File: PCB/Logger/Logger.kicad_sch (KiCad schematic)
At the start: 78 parts, among them J2 USB-C-Socket-V, J3 JST-PH-SM4-TB, J4 Reset, J5 Conn_01x05, J6 TF_PUSH, J7 TC2030-USB-NL-DS, Q1 C179347, Q4 CJ2301, U1 TP4054, U10 ESP32-S3-MINI-1, U2 ME6211C33M5G-N

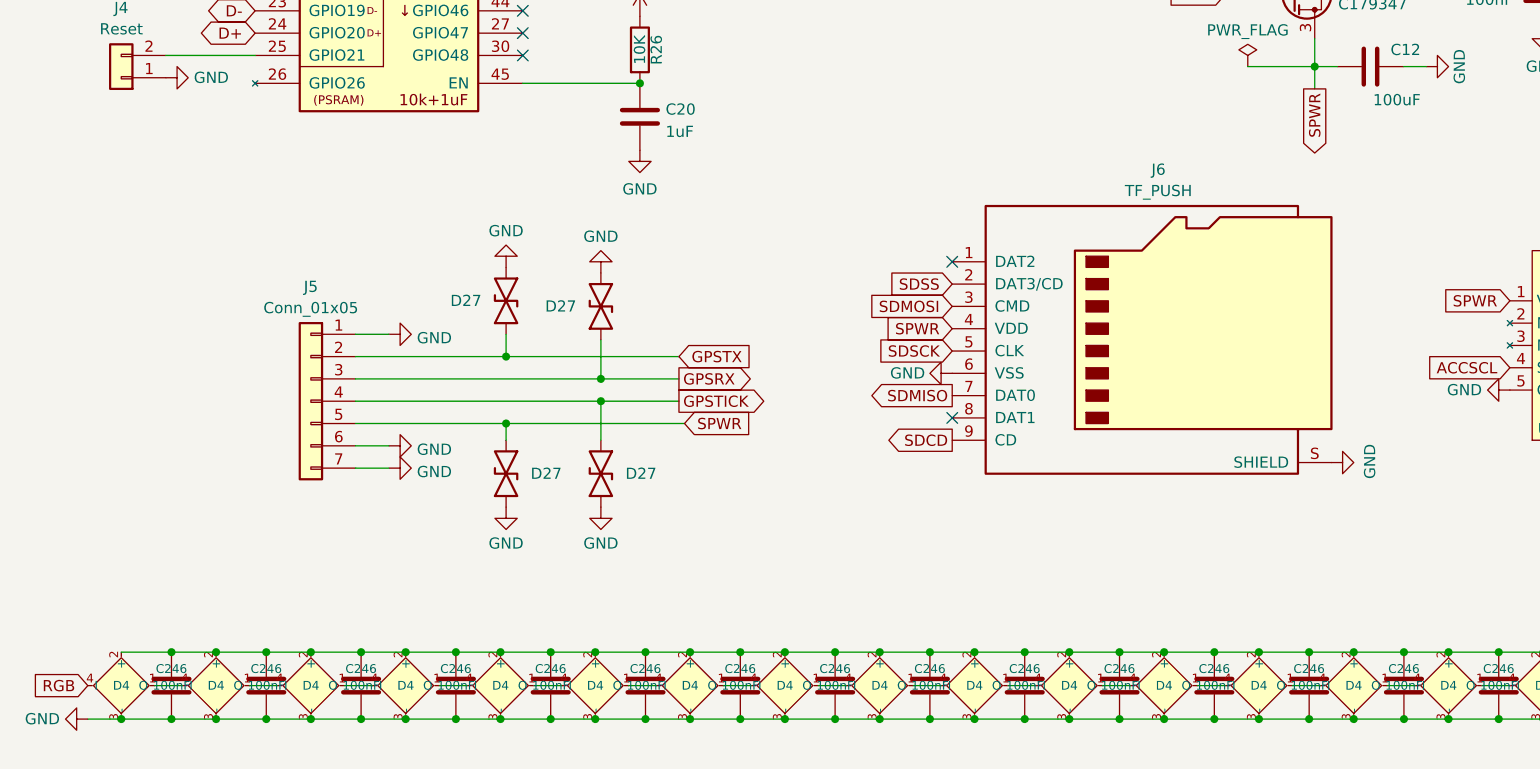
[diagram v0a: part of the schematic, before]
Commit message: Resistors
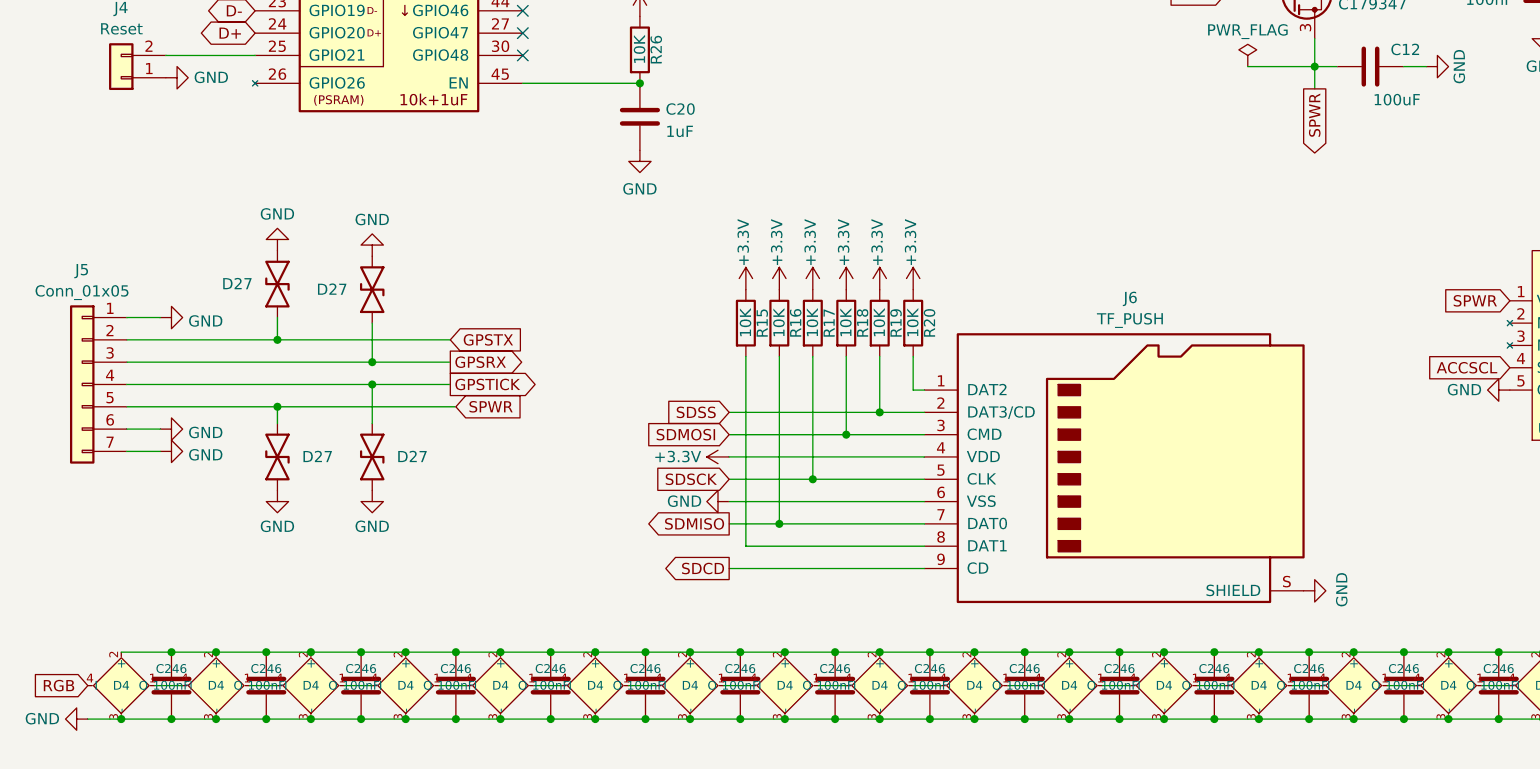
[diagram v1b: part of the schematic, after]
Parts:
- added R15, R16, R17, R18, R19, R20: 10K, RevK:R_0402, symbol Device:R
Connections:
- net +3.3V: now also J6.4 (VDD), R15.1, R16.1, R17.1, R18.1, R19.1, R20.1
- net SDMISO: now also R16.2
- net SDMOSI: now also R18.2
- net SDSCK: now also R17.2
- net SDSS: now also R19.2
- net SPWR: no longer J6.4 (VDD)
- net at J6.1 (DAT2): now also R20.2
- net at J6.8 (DAT1): now also R15.2
- no-connect marks 24 -> 22
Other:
- moved on the sheet: D27, J5, J6
